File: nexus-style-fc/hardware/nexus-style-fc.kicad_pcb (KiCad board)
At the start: 4 copper layers, 22.4 x 33.1 mm, 88 parts, among them J1 Header child board, J2 DSM (UART1), J3 A-CRSF (UART4), J4 C (UART3), J5 B (UART6), J6 USB-C vertical, SW1 BOOT, U1 STM32F722RET6, U10 TPS70933DBVR, U11 SRV05-4, U12 SRV05-4, U13 SRV05-4, U14 TPS629210DRLR, U15 SRV05-4, U2 ICM-42688-P, U3 DPS368XTSA1, U4 W25N01GVZEIG, U5 TPS62130RGTR, U7 USBLC6-2SC6, U9 TPS2116DRLR, Y1 8MHz 20pF

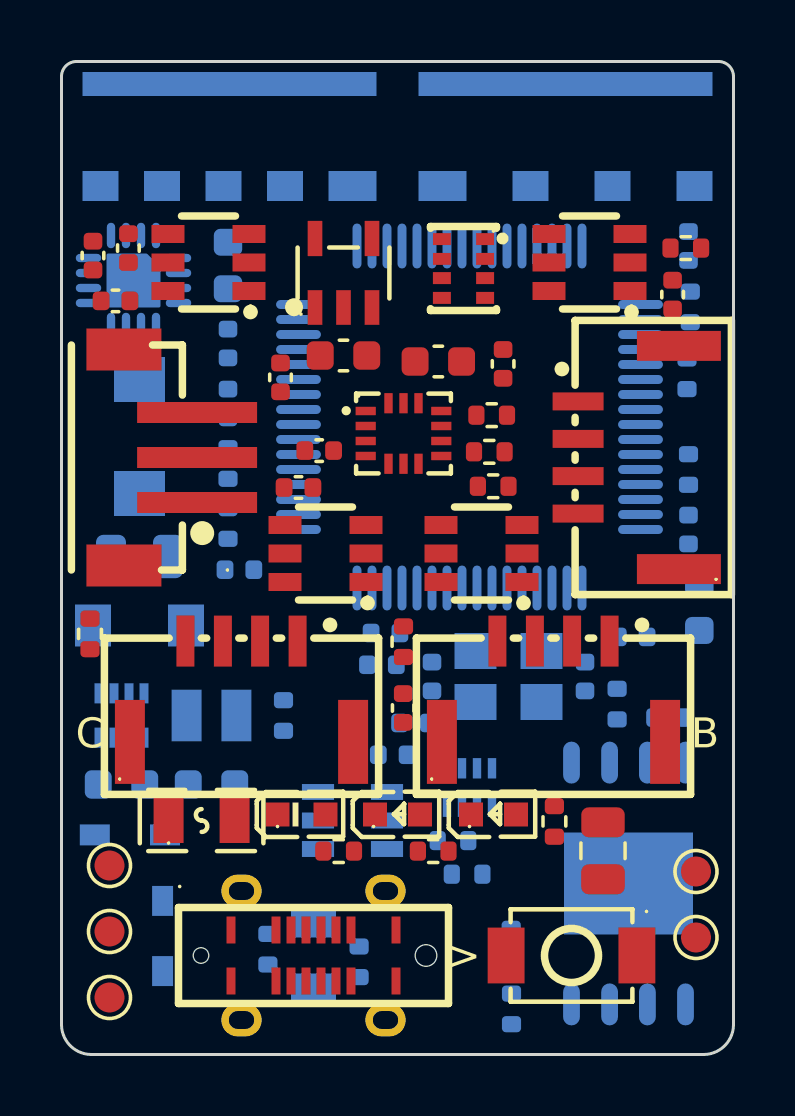
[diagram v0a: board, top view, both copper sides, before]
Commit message: cleaned up the nets
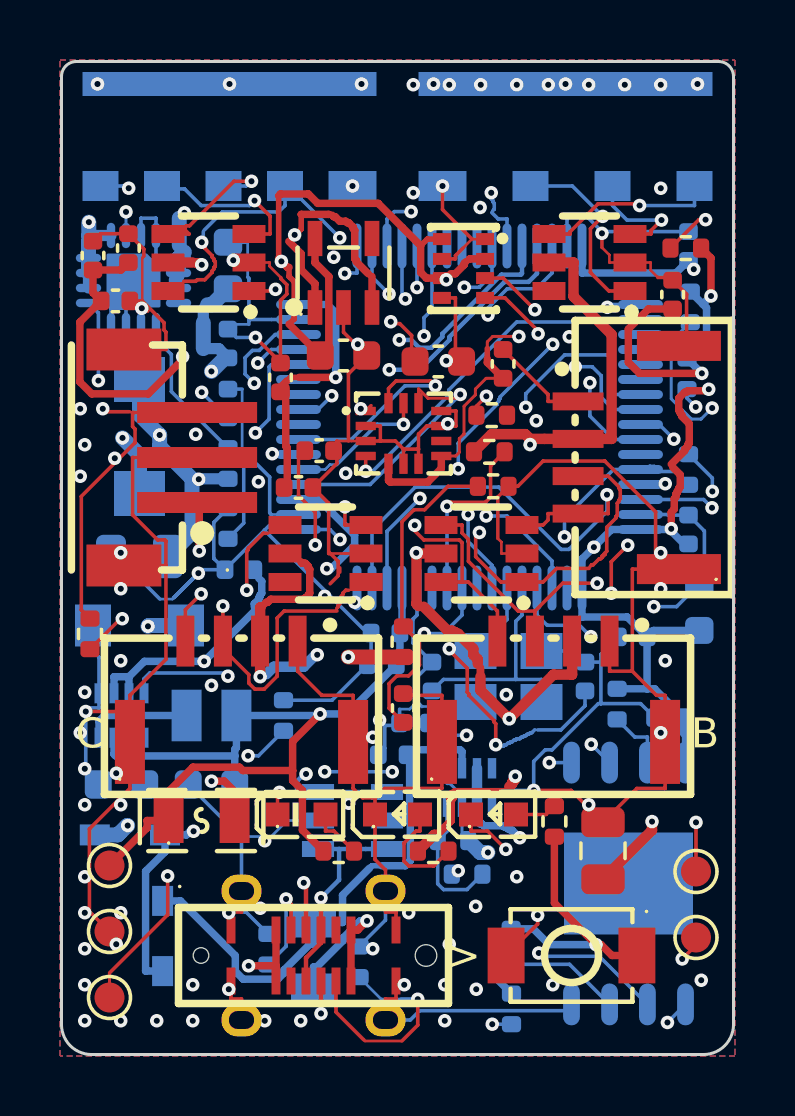
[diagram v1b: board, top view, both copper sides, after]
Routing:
- net GND: track 0.00 -> 230.6 mm, vias 0 -> 75
- net 3V3: track 0.00 -> 125.0 mm, vias 0 -> 8
- net VX: track 0.00 -> 85.3 mm, vias 0 -> 9
- net 5V: track 0.00 -> 81.0 mm, vias 0 -> 9
- net 3V3_SENS: track 0.00 -> 64.7 mm, vias 0 -> 6
- net DSM_DATA: track 0.00 -> 61.2 mm, vias 0 -> 6
- net VSYS: track 0.00 -> 49.4 mm, vias 0 -> 3
- net NRST: track 0.00 -> 43.9 mm, vias 0 -> 3
- net 5V_BUCK: track 0.00 -> 39.8 mm, vias 0 -> 4
- net USB_DP: track 0.00 -> 37.9 mm, vias 0 -> 5
- net DSM_TX: track 0.00 -> 37.5 mm, vias 0 -> 6
- net FLASH_CS: track 0.00 -> 36.4 mm, vias 0 -> 3
- net SPI2_MISO: track 0.00 -> 33.7 mm, vias 0 -> 2
- net SWCLK: track 0.00 -> 33.6 mm, vias 0 -> 2
- net USB_DM: track 0.00 -> 33.1 mm, vias 0 -> 2
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- added copper zone on B.Cu, net GND
- added copper zone on F.Cu, net GND
- added copper zone on In1.Cu, net GND
- added copper zone on In2.Cu, net GND
- added copper zone on In3.Cu, net GND
- added copper zone on In4.Cu, net GND
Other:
- copper layers 4 -> 6

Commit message: tidied up the nets
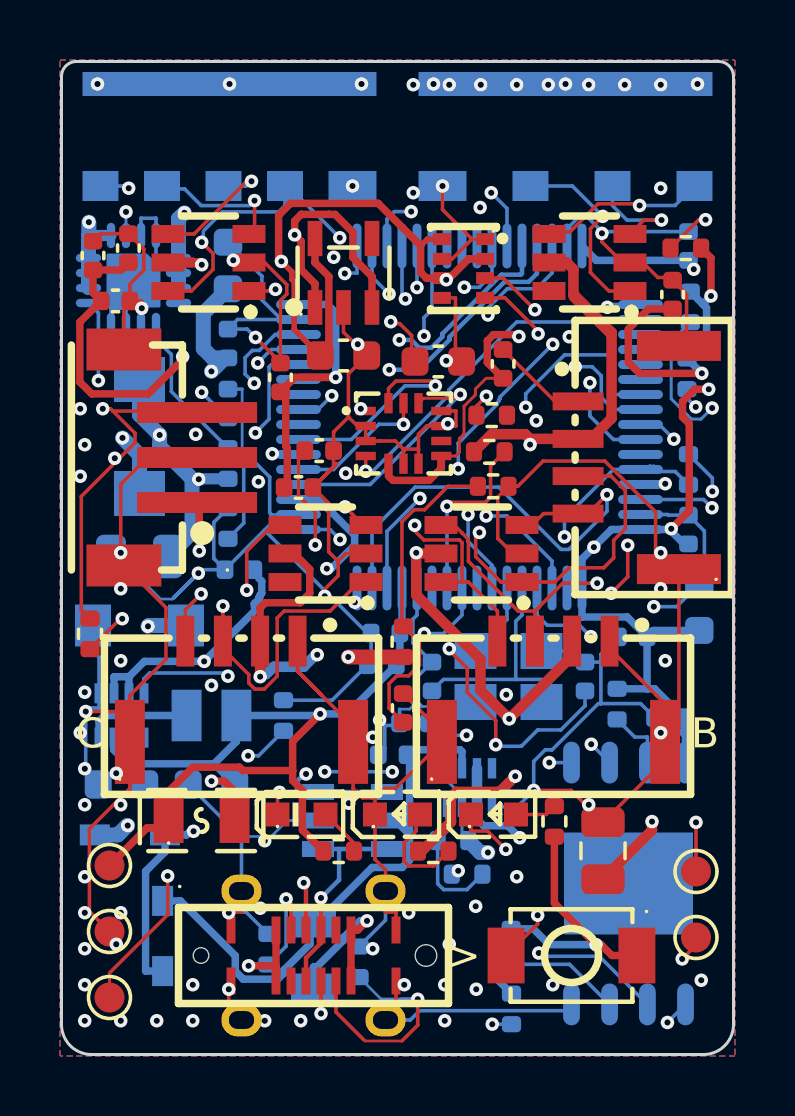
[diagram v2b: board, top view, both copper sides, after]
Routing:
- net GND: track 230.6 -> 227.4 mm
- net 5V: track 81.0 -> 83.2 mm
- net DSM_DATA: track 61.2 -> 62.2 mm
- net SW_5V: track 12.2 -> 13.0 mm
- net RPM: track 21.0 -> 20.1 mm
- net TAIL: track 23.1 -> 23.8 mm
- net A_TX: track 16.1 -> 15.4 mm
- net C_RX: track 18.6 -> 19.2 mm

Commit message: tidied up the nets
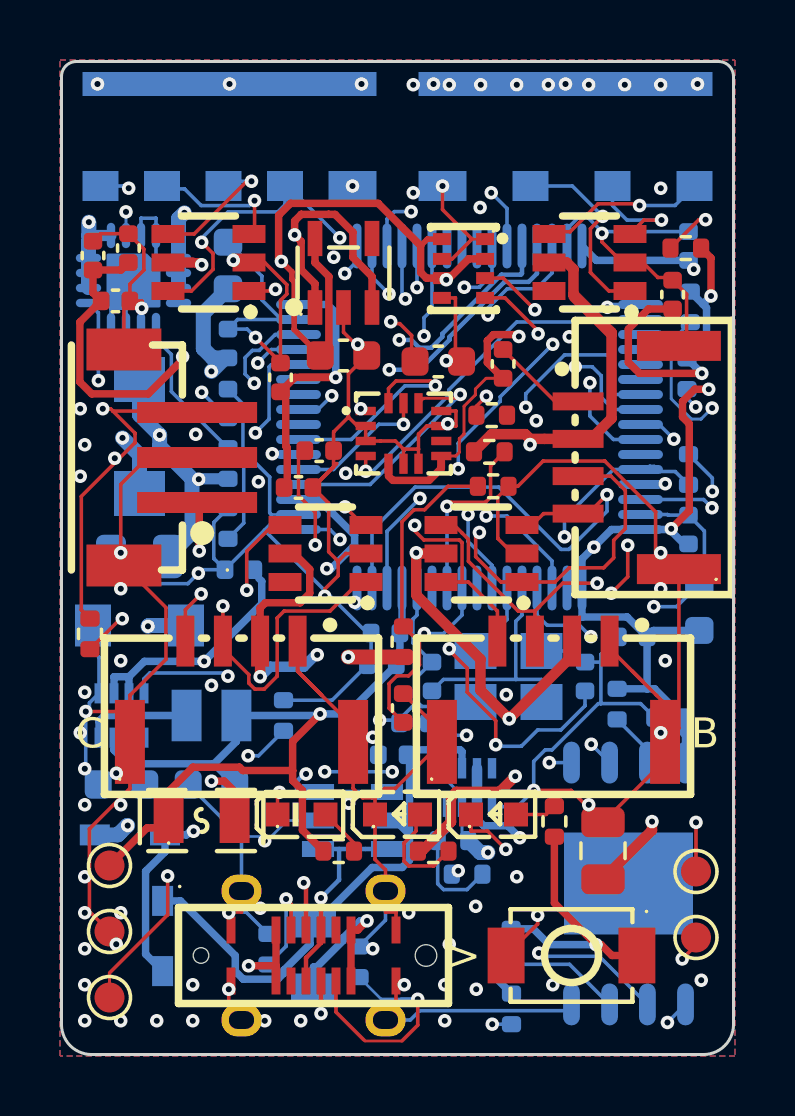
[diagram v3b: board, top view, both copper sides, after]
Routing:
- net VX: track 85.7 -> 100.1 mm
- net GND: track 227.4 -> 225.1 mm
- net 3V3: track 125.1 -> 126.0 mm
- net 5V: track 83.2 -> 84.0 mm
- net USB_DP: track 37.9 -> 37.2 mm
- net I2C1_SCL: track 16.8 -> 17.4 mm
- net NRST: track 43.9 -> 44.5 mm
